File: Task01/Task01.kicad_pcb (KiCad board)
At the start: 2 copper layers, 55.5 x 32 mm, 28 parts, among them J1 Conn_01x02_Pin, J3 DC, J4 DC, Q1 BC547, U1 NE555P

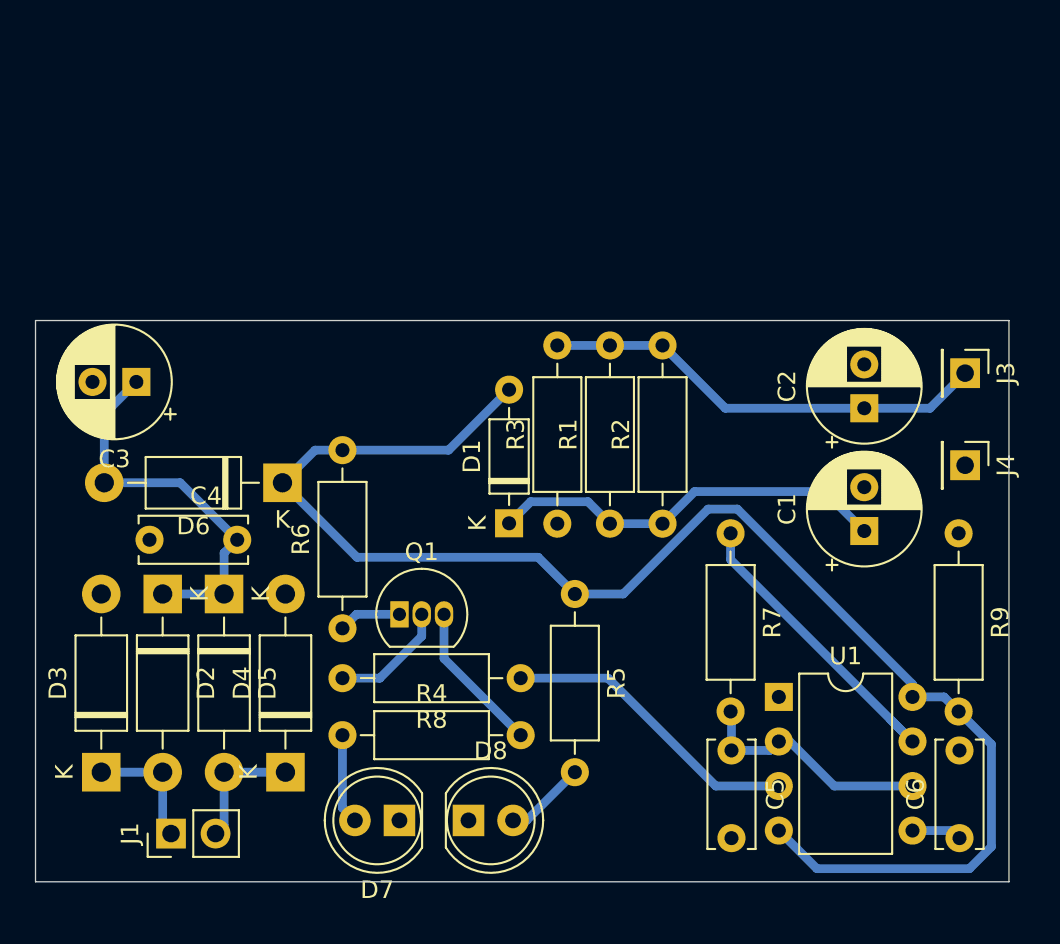
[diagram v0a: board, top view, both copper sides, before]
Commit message: will add gitignore later
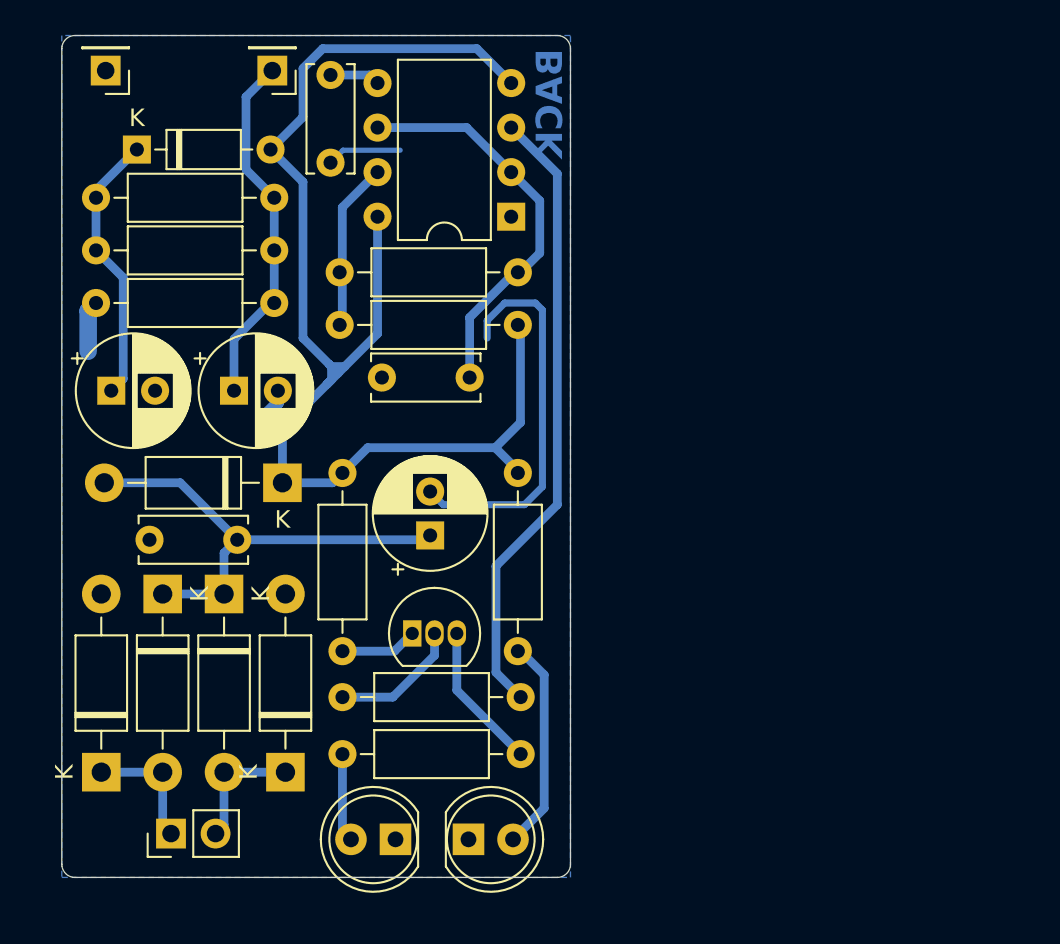
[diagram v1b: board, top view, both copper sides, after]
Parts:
- moved C6 56.4 mm to (176.3, 44.0), turned to -90 degrees
- moved J4 53.9 mm to (163.5, 43.8), turned to 180 degrees
- moved C1 43.7 mm to (163.8, 62.0), turned to 0 degrees
- moved J3 43.1 mm to (173.0, 43.8), turned to 180 degrees
- moved R2 37.3 mm to (162.9, 51.0), turned to 0 degrees
- moved R9 37.2 mm to (176.8, 58.2), turned to 0 degrees
- moved C2 35.9 mm to (170.8, 62.0), turned to 0 degrees
- moved R1 33.2 mm to (162.9, 54.0), turned to 0 degrees
- moved U1 31.3 mm to (186.6, 52.1), turned to 180 degrees
- moved D1 30.1 mm to (165.3, 48.2), turned to 0 degrees
- moved R3 29.2 mm to (162.9, 57.0), turned to 0 degrees
- moved R7 26.8 mm to (176.8, 55.2), turned to 0 degrees
- moved C5 26.0 mm to (184.2, 61.2), turned to 180 degrees
- moved C3 18.9 mm to (182.0, 70.2), turned to 90 degrees
- moved R5 7.63 mm to (187.0, 66.7)
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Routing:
- net GND: track 0.00 -> 31.0 mm
- net Net-(U1-Q): track 17.6 -> 35.6 mm
- net VCC: track 85.5 -> 75.6 mm
- net TR: track 13.8 -> 22.9 mm
- net DIS: track 17.9 -> 9.54 mm
- net Net-(D8-A): track 4.66 -> 12.0 mm
- net Net-(D1-K): track 23.0 -> 15.6 mm
- net DC_OUT: track 25.6 -> 20.6 mm
- net VCCQ: track 22.3 -> 26.9 mm
- net Net-(Q1-C): track 3.58 -> 4.40 mm
- net BCE: track 6.76 -> 7.49 mm
- added copper zone on B.Cu, net GND
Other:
- board size 55.5 x 32 mm -> 29 x 48 mm
- board text added: "BACK"
